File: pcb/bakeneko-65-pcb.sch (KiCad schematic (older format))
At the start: 17 parts, among them J1 JST SH 4-pin, SW1 Reset, U1 USBLC6-2SC6, U2 ATmega32U4-AU, Y1 16MHz

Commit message: yep
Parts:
- added AdafruitLEBluetooth1: Conn_01x09_MountingPin, Connector_PinHeader_2.54mm:PinHeader_1x09_P2.54mm_Vertical, symbol Connector_Generic_MountingPin:Conn_01x09_MountingPin
- U1: symbol Power_Protection:USBLC6-2SC6 -> bakeneko-65-pcb-rescue:USBLC6-2SC6-Power_Protection
- U2: symbol MCU_Microchip_ATmega:ATmega32U4-AU -> bakeneko-65-pcb-rescue:ATmega32U4-AU-MCU_Microchip_ATmega
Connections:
- net labels added: BleCS, BleIRQ, BleReset
- wire segments 40 -> 44
- no-connect marks 5 -> 2
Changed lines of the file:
@@
 EESchema Schematic File Version 4
-LIBS:bakeneko-65-pcb-cache
 EELAYER 30 0
 EELAYER END
@@
 D+
 $Comp
-L MCU_Microchip_ATmega:ATmega32U4-AU U2
+L bakeneko-65-pcb-rescue:ATmega32U4-AU-MCU_Microchip_ATmega U2
 U 1 1 5F26004F
 P 2350 5400
@@
 ROW2
 $Comp
-L Power_Protection:USBLC6-2SC6 U1
+L bakeneko-65-pcb-rescue:USBLC6-2SC6-Power_Protection U1
 U 1 1 5F25444E
 P 4550 1700
@@
 Text GLabel 2950 6500 2    50   Input ~ 0
 ROW3
-NoConn ~ 2950 4000
-NoConn ~ 2950 4100
-NoConn ~ 2950 4200
+Text GLabel 2950 4000 2    50   Input ~ 0
+BleReset
+Text GLabel 2950 4100 2    50   Input ~ 0
+BleCS
+Text GLabel 2950 4200 2    50   Input ~ 0
+BleIRQ
+$Comp
+L Connector_Generic_MountingPin:Conn_01x09_MountingPin AdafruitLEBluetooth1
+U 1 1 60AA66F6
+P 6950 1950
+F 0 "AdafruitLEBluetooth1" H 7038 1914 50  0000 L CNN
+F 1 "Conn_01x09_MountingPin" H 7038 1823 50  0000 L CNN
+F 2 "Connector_PinHeader_2.54mm:PinHeader_1x09_P2.54mm_Vertical" H 6950 1950 50  0001 C CNN
+F 3 "~" H 6950 1950 50  0001 C CNN
+	1    6950 1950
+	1    0    0    -1
+$EndComp
+Text GLabel 6750 1850 0    50   Input ~ 0
+BleCS
+Text GLabel 6750 1950 0    50   Input ~ 0
+BleIRQ
+Text GLabel 6750 2150 0    50   Input ~ 0
+BleReset
+$Comp
+L power:GND #PWR?
+U 1 1 60AA59B8
+P 6650 2250
+F 0 "#PWR?" H 6650 2000 50  0001 C CNN
+F 1 "GND" H 6655 2077 50  0000 C CNN
+F 2 "" H 6650 2250 50  0001 C CNN
+F 3 "" H 6650 2250 50  0001 C CNN
+	1    6650 2250
+	1    0    0    -1
+$EndComp
+Wire Wire Line
+	6750 2250 6650 2250
+$Comp
+L power:+5V #PWR?
+U 1 1 60AA8156
+P 6500 2350
+F 0 "#PWR?" H 6500 2200 50  0001 C CNN
+F 1 "+5V" H 6515 2523 50  0000 C CNN
+F 2 "" H 6500 2350 50  0001 C CNN
+F 3 "" H 6500 2350 50  0001 C CNN
+	1    6500 2350
+	1    0    0    -1
+$EndComp
+Wire Wire Line
+	6750 2400 6500 2400
+Wire Wire Line
+	6500 2350 6500 2400
+Wire Wire Line
+	6750 2400 6750 2350
 $EndSCHEMATC

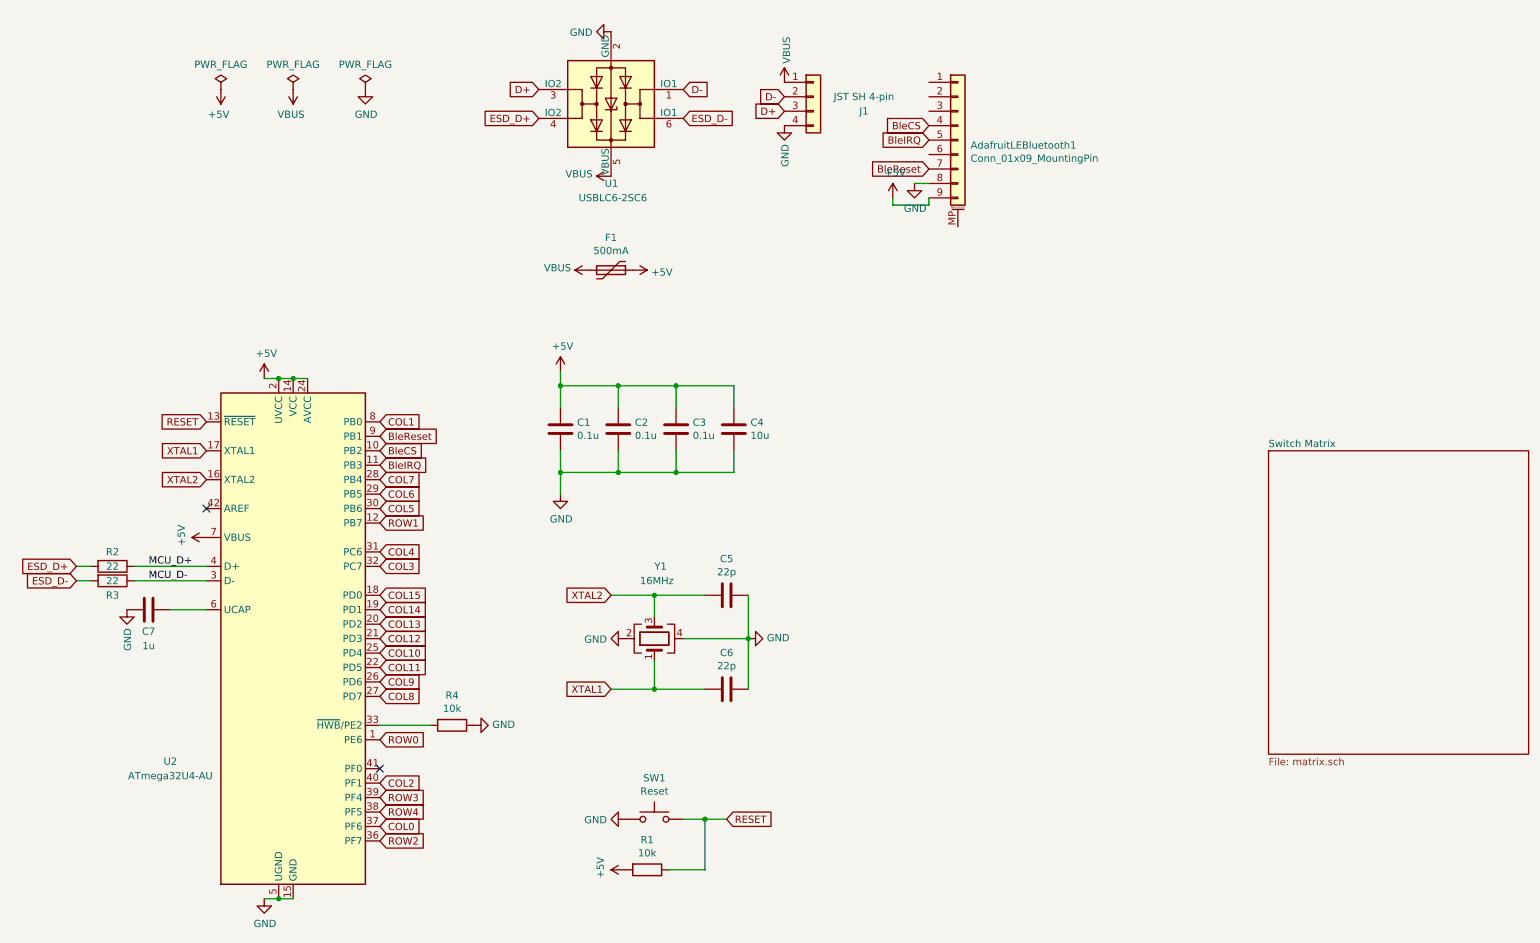
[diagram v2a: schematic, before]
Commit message: finished keyboard pcb
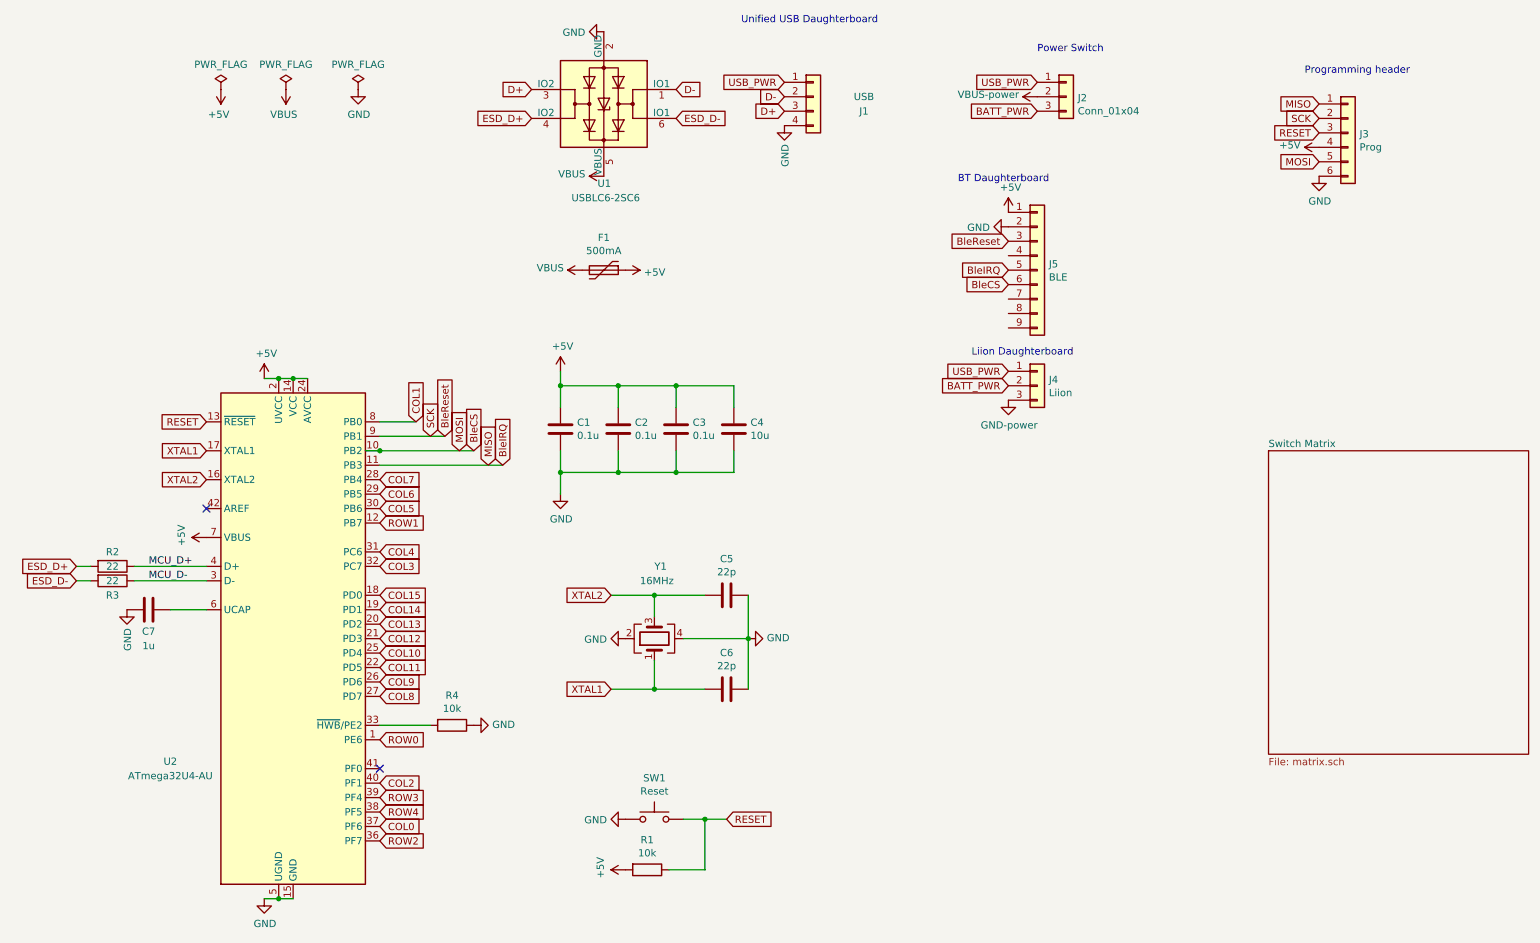
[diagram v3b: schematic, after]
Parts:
- removed AdafruitLEBluetooth1: Conn_01x09_MountingPin, Connector_PinHeader_2.54mm:PinHeader_1x09_P2.54mm_Vertical, symbol Connector_Generic_MountingPin:Conn_01x09_MountingPin
- added J2: Conn_01x04, Connector_JST:JST_SH_BM03B-SRSS-TB_1x03-1MP_P1.00mm_Vertical, symbol Connector_Generic:Conn_01x03
- added J3: Prog, Connector_PinHeader_2.54mm:PinHeader_1x06_P2.54mm_Vertical, symbol Connector_Generic:Conn_01x06
- added J4: Liion, Connector_JST:JST_SH_BM03B-SRSS-TB_1x03-1MP_P1.00mm_Vertical, symbol Connector_Generic:Conn_01x03
- added J5: BLE, Connector_PinHeader_2.54mm:PinHeader_1x09_P2.54mm_Vertical, symbol Connector_Generic:Conn_01x09
- J1: value JST SH 4-pin -> USB
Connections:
- net +5V: now also J3.4 (Pin_4), J5.1 (Pin_1)
- net BleCS: now also J3.5 (Pin_5), J5.6 (Pin_6)
- net BleIRQ: now also J3.1 (Pin_1), J5.5 (Pin_5)
- net BleReset: now also J3.2 (Pin_2), J5.3 (Pin_3)
- net GND: now also J3.6 (Pin_6), J4.3 (Pin_3), J5.2 (Pin_2)
- net RESET: now also J3.3 (Pin_3)
- net VBUS: now also J2.2 (Pin_2); no longer J1.1 (Pin_1)
- new net BATT_PWR: J2.3 (Pin_3), J4.2 (Pin_2)
- new net USB_PWR: J1.1 (Pin_1), J2.1 (Pin_1), J4.1 (Pin_1)
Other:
- note added: "BT Daughterboard\n"
- note added: "Liion Daughterboard"
- note added: "Power Switch"
- note added: "Programming header\n"
- note added: "Unified USB Daughterboard\n"
- moved on the sheet: F1, U1
